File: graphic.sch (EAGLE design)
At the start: 81 parts, among them IC1 NE5532D, IC2 NE5532D, IC3 NE5532D, IC4 NE5532D, IC5 NE5532D

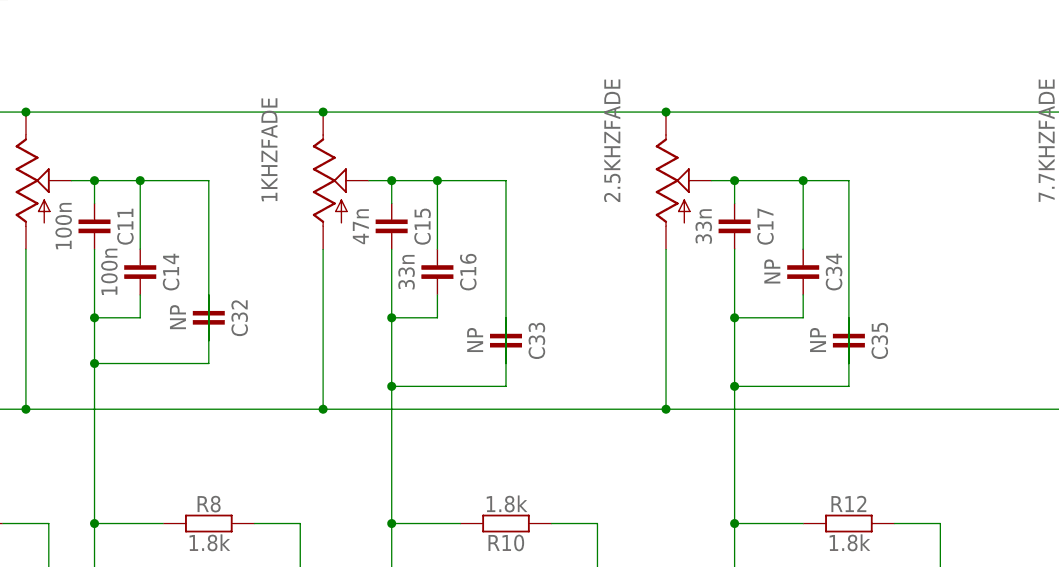
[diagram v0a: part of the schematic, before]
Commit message: re route and redesign panel
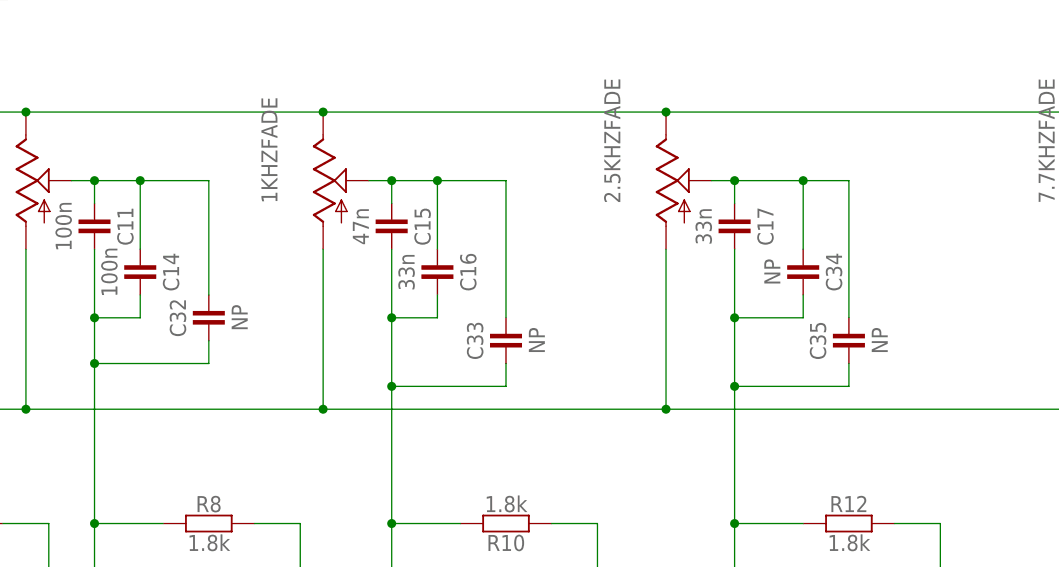
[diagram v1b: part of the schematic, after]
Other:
- moved on the sheet: C32, C33, C35
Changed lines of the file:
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@@
 <instance part="IC5" gate="A" x="322.58" y="88.9"/>
 <instance part="C31" gate="C" x="88.9" y="114.3" rot="R270"/>
-<instance part="C32" gate="C" x="119.38" y="114.3" rot="R270"/>
-<instance part="C33" gate="C" x="152.4" y="111.76" rot="R270"/>
+<instance part="C32" gate="C" x="119.38" y="114.3" rot="R90"/>
+<instance part="C33" gate="C" x="152.4" y="111.76" rot="R90"/>
 <instance part="C34" gate="C" x="185.42" y="119.38" rot="R270"/>
-<instance part="C35" gate="C" x="190.5" y="111.76" rot="R270"/>
+<instance part="C35" gate="C" x="190.5" y="111.76" rot="R90"/>
 <instance part="C36" gate="C" x="236.22" y="111.76" rot="R270"/>
 <instance part="C37" gate="C" x="284.48" y="121.92" rot="R270"/>
@@
 <junction x="106.68" y="129.54"/>
 <pinref part="C32" gate="C" pin="2"/>
-<wire x1="119.38" y1="111.76" x2="119.38" y2="129.54" width="0.1524" layer="91"/>
+<wire x1="119.38" y1="116.84" x2="119.38" y2="129.54" width="0.1524" layer="91"/>
 <wire x1="119.38" y1="129.54" x2="111.76" y2="129.54" width="0.1524" layer="91"/>
 <junction x="111.76" y="129.54"/>
@@
 <pinref part="1KHZ" gate="FADE" pin="S"/>
 <pinref part="C33" gate="C" pin="2"/>
-<wire x1="152.4" y1="109.22" x2="152.4" y2="129.54" width="0.1524" layer="91"/>
+<wire x1="152.4" y1="114.3" x2="152.4" y2="129.54" width="0.1524" layer="91"/>
 <wire x1="152.4" y1="129.54" x2="144.78" y2="129.54" width="0.1524" layer="91"/>
 <junction x="144.78" y="129.54"/>
@@
 <junction x="177.8" y="129.54"/>
 <pinref part="C35" gate="C" pin="2"/>
-<wire x1="190.5" y1="109.22" x2="190.5" y2="129.54" width="0.1524" layer="91"/>
+<wire x1="190.5" y1="114.3" x2="190.5" y2="129.54" width="0.1524" layer="91"/>
 <wire x1="190.5" y1="129.54" x2="185.42" y2="129.54" width="0.1524" layer="91"/>
 <junction x="185.42" y="129.54"/>
@@
 <pinref part="C32" gate="C" pin="1"/>
 <wire x1="106.68" y1="109.22" x2="106.68" y2="114.3" width="0.1524" layer="91"/>
-<wire x1="119.38" y1="116.84" x2="119.38" y2="109.22" width="0.1524" layer="91"/>
+<wire x1="119.38" y1="111.76" x2="119.38" y2="109.22" width="0.1524" layer="91"/>
 <wire x1="119.38" y1="109.22" x2="106.68" y2="109.22" width="0.1524" layer="91"/>
 <junction x="106.68" y="109.22"/>
@@
 <pinref part="C33" gate="C" pin="1"/>
 <wire x1="139.7" y1="106.68" x2="139.7" y2="114.3" width="0.1524" layer="91"/>
-<wire x1="152.4" y1="114.3" x2="152.4" y2="106.68" width="0.1524" layer="91"/>
+<wire x1="152.4" y1="109.22" x2="152.4" y2="106.68" width="0.1524" layer="91"/>
 <wire x1="152.4" y1="106.68" x2="139.7" y2="106.68" width="0.1524" layer="91"/>
 <junction x="139.7" y="106.68"/>
@@
 <junction x="177.8" y="114.3"/>
 <pinref part="C35" gate="C" pin="1"/>
-<wire x1="190.5" y1="114.3" x2="190.5" y2="106.68" width="0.1524" layer="91"/>
+<wire x1="190.5" y1="109.22" x2="190.5" y2="106.68" width="0.1524" layer="91"/>
 <wire x1="190.5" y1="106.68" x2="177.8" y2="106.68" width="0.1524" layer="91"/>
 <junction x="177.8" y="106.68"/>
